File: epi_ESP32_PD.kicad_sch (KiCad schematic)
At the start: 62 parts, among them J1 Conn_01x08, J2 USB_C_Receptacle_USB2.0, J3 Conn_01x08, J4 Conn_01x01, J6 Conn_Coaxial_Small, J7 Conn_02x03, J8 Conn_01x03, Q1 Q_PMOS_GDS, Q2 Q_NMOS_GDS, Q3 Q_NMOS_GDS, Q4 Q_NMOS_GDS, Q5 Q_NMOS_GDS, Q6 Q_NMOS_GDS, SW1 SW_MEC_5G, SW2 SW_MEC_5G, U1 ESP32-C3, U2 MIC5219-3.3YM5, U5 AP63205WU, Y1 Crystal

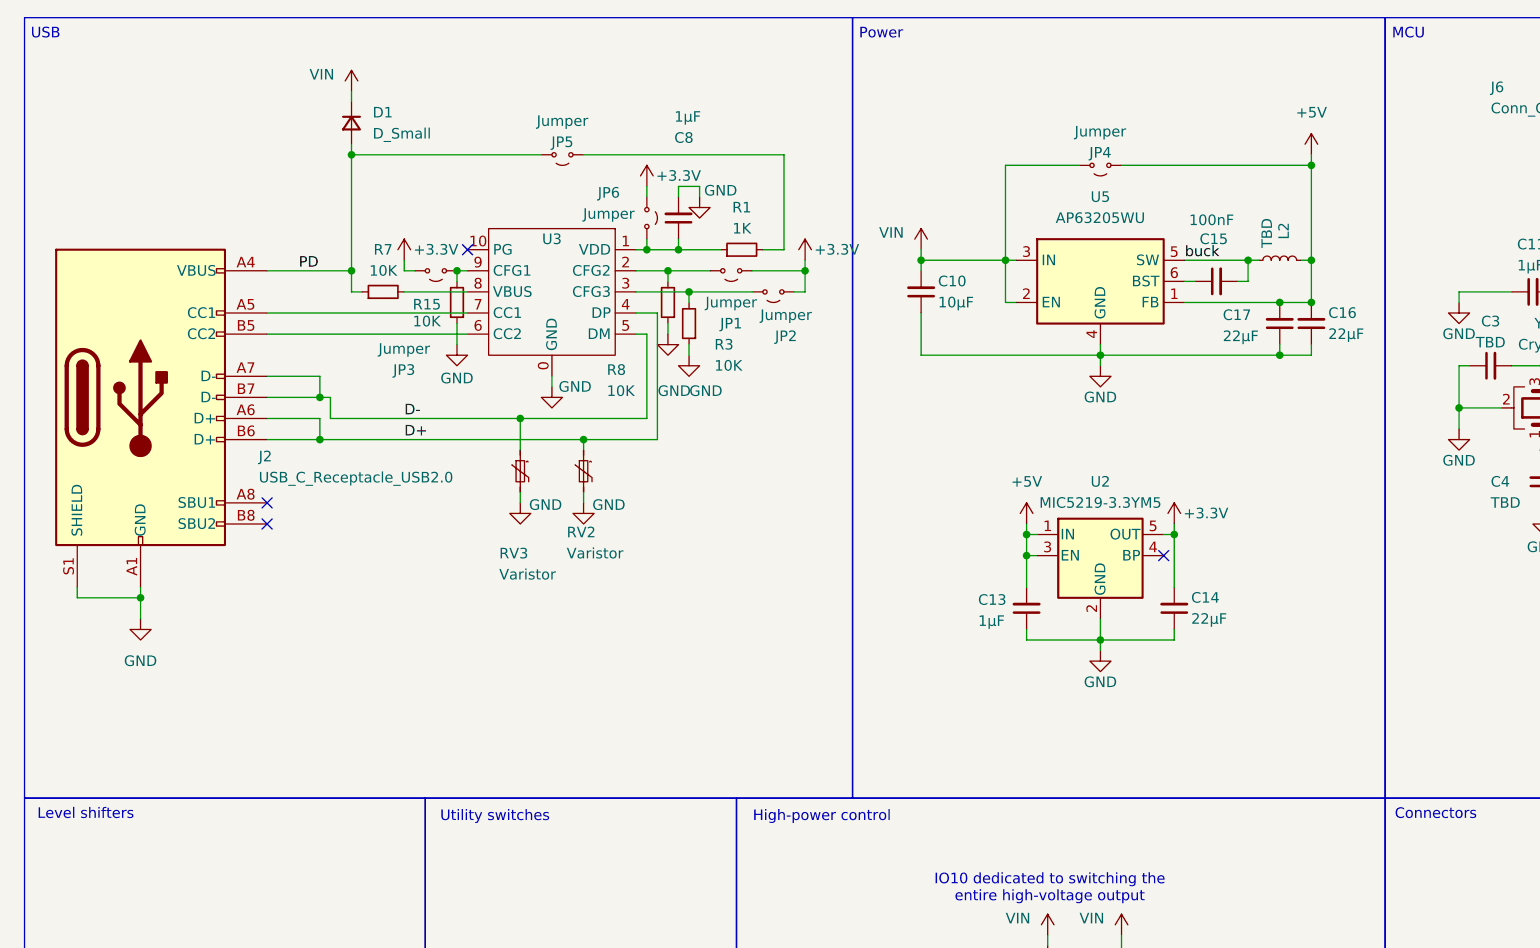
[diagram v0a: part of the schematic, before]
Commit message: mix
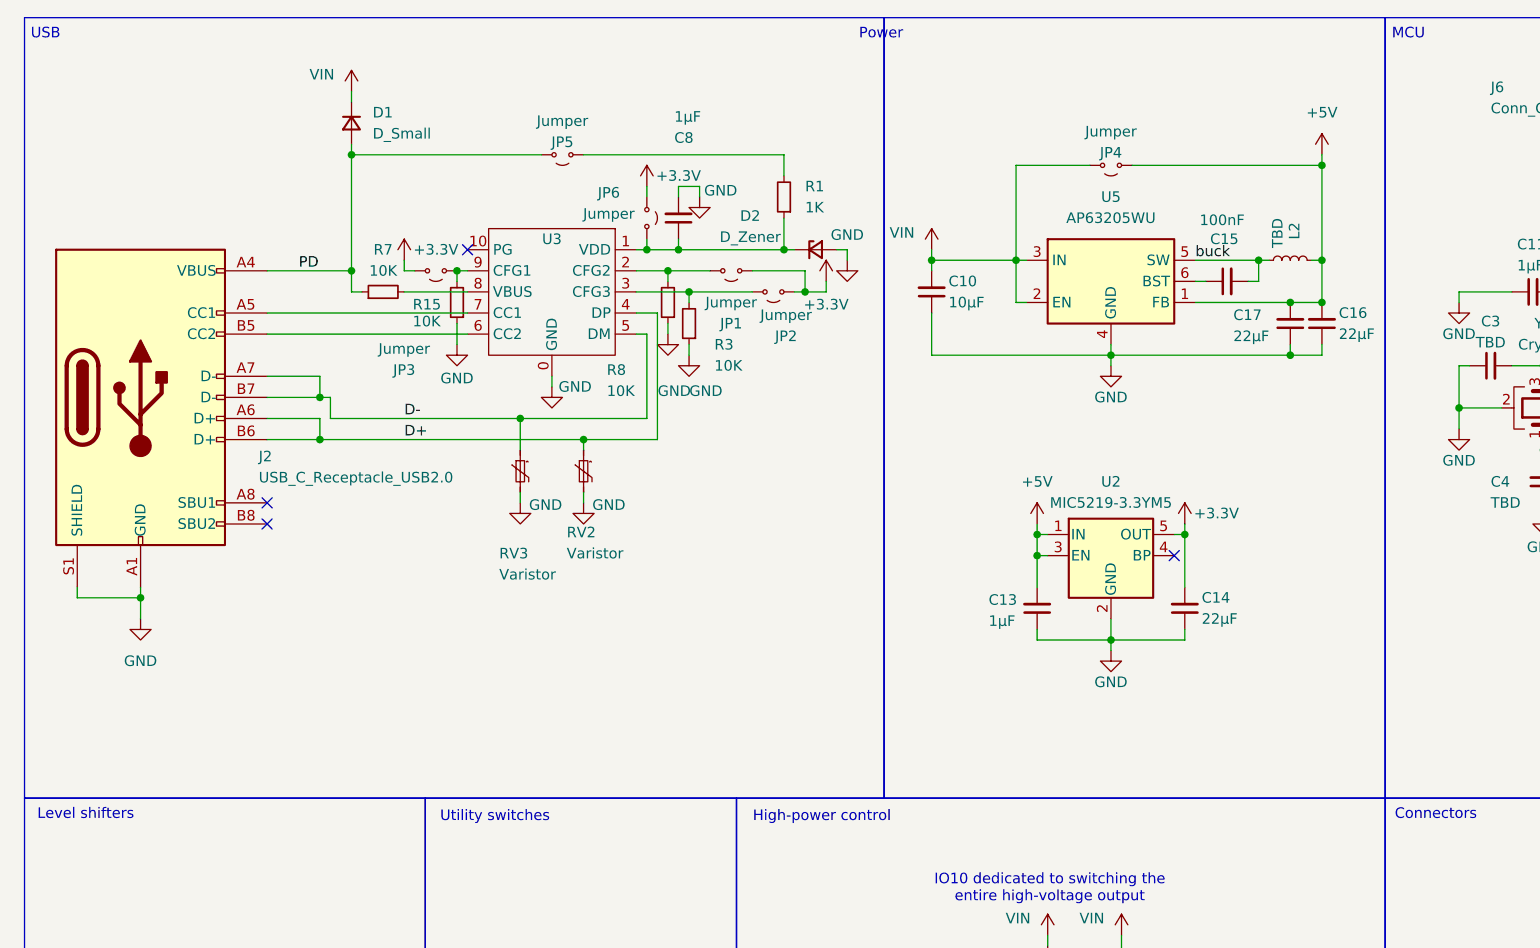
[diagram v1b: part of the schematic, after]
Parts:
- added D2: D_Zener, Diode_SMD:D_SOD-323, symbol Device:D_Zener_Small
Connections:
- net GND: now also D2.2 (A)
- net at C8.1, JP6.2 (B), R1.1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: now also D2.1 (K)
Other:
- moved on the sheet: C10, C13, C14, C15, C16, C17, JP4, L2, R1, U2, U5
